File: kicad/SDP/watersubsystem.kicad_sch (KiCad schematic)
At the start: 6 parts

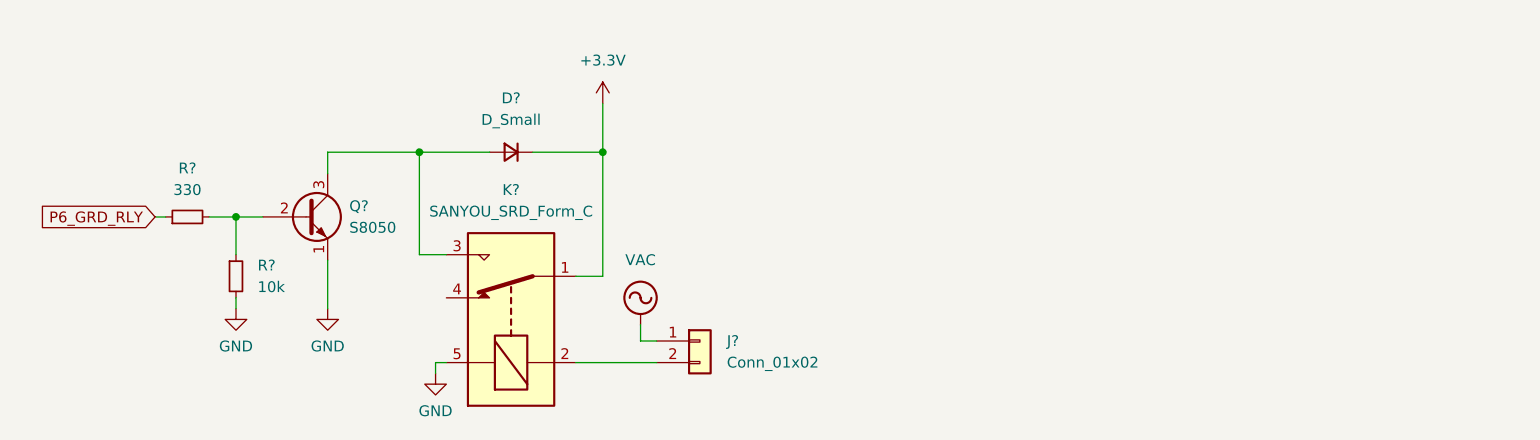
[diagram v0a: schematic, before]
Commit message: Updated schematics
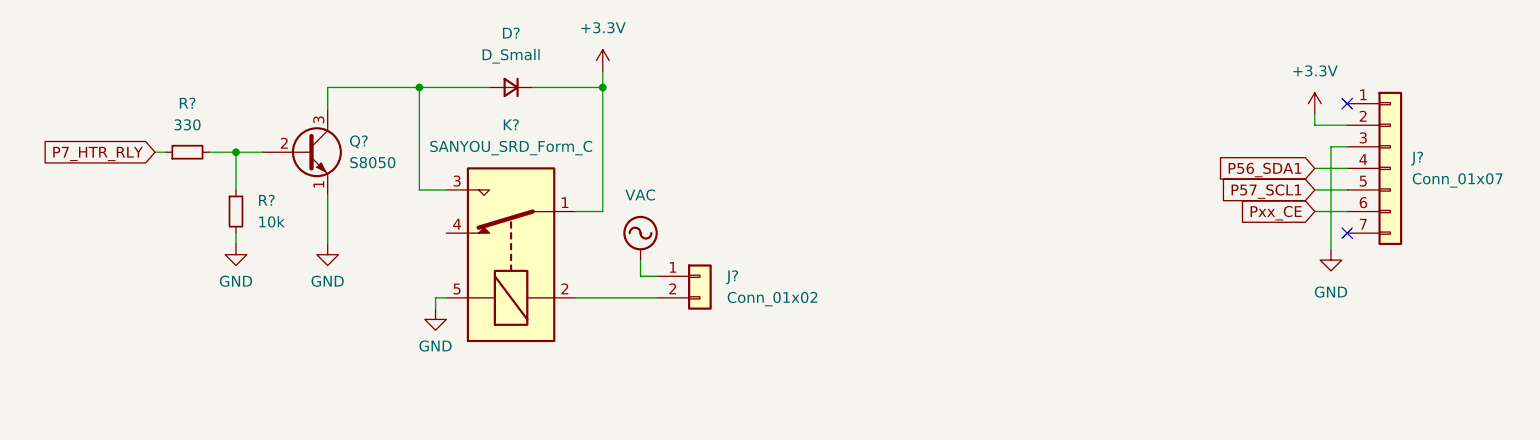
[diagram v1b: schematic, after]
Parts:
- removed D?: D_Small, symbol Device:D_Small
- removed J?: Conn_01x02, symbol Connector_Generic:Conn_01x02
- removed K?: SANYOU_SRD_Form_C, Relay_THT:Relay_SPDT_SANYOU_SRD_Series_Form_C, symbol Relay:SANYOU_SRD_Form_C
- removed Q?: S8050, Package_TO_SOT_THT:TO-92_Inline, symbol Transistor_BJT:S8050
- removed R?: 10k, symbol Device:R_Small
- removed R?: 330, symbol Device:R_Small
- added D?: D_Small, symbol Device:D_Small
- added J?: Conn_01x02, symbol Connector_Generic:Conn_01x02
- added J?: Conn_01x07, symbol Connector_Generic:Conn_01x07
- added K?: SANYOU_SRD_Form_C, Relay_THT:Relay_SPDT_SANYOU_SRD_Series_Form_C, symbol Relay:SANYOU_SRD_Form_C
- added Q?: S8050, Package_TO_SOT_THT:TO-92_Inline, symbol Transistor_BJT:S8050
- added R?: 330, symbol Device:R_Small
- added R?: 10k, symbol Device:R_Small
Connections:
- net +3V3: now also D?.1 (K), J?.2 (Pin_2), K?.1
- net GND: now also J?.3 (Pin_3), K?.5, Q?.1 (E), R?.2
- net VAC: now also J?.1 (Pin_1)
- new net: Q?.2 (B), R?.1, R?.2
- new net: D?.2 (A), K?.3, Q?.3 (C)
- new net: J?.2 (Pin_2), K?.2
- new net P56_SDA1: J?.4 (Pin_4)
- new net P57_SCL1: J?.5 (Pin_5)
- new net P7_HTR_RLY: R?.1
- new net Pxx_CE: J?.6 (Pin_6)
- no-connect marks 0 -> 2

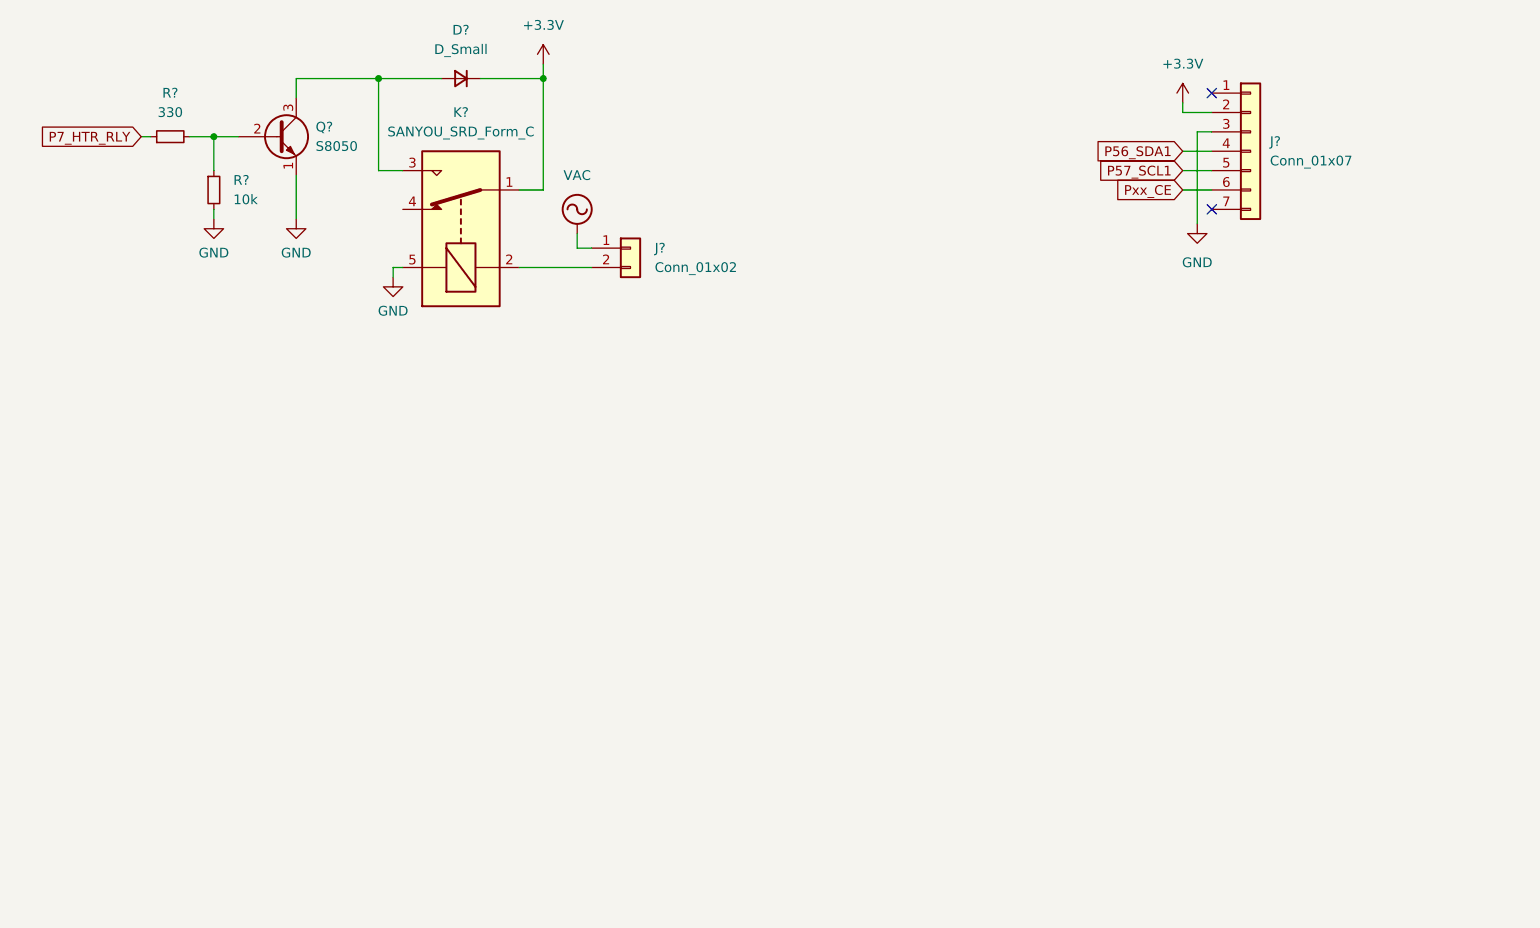
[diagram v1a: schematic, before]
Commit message: Updated schematics
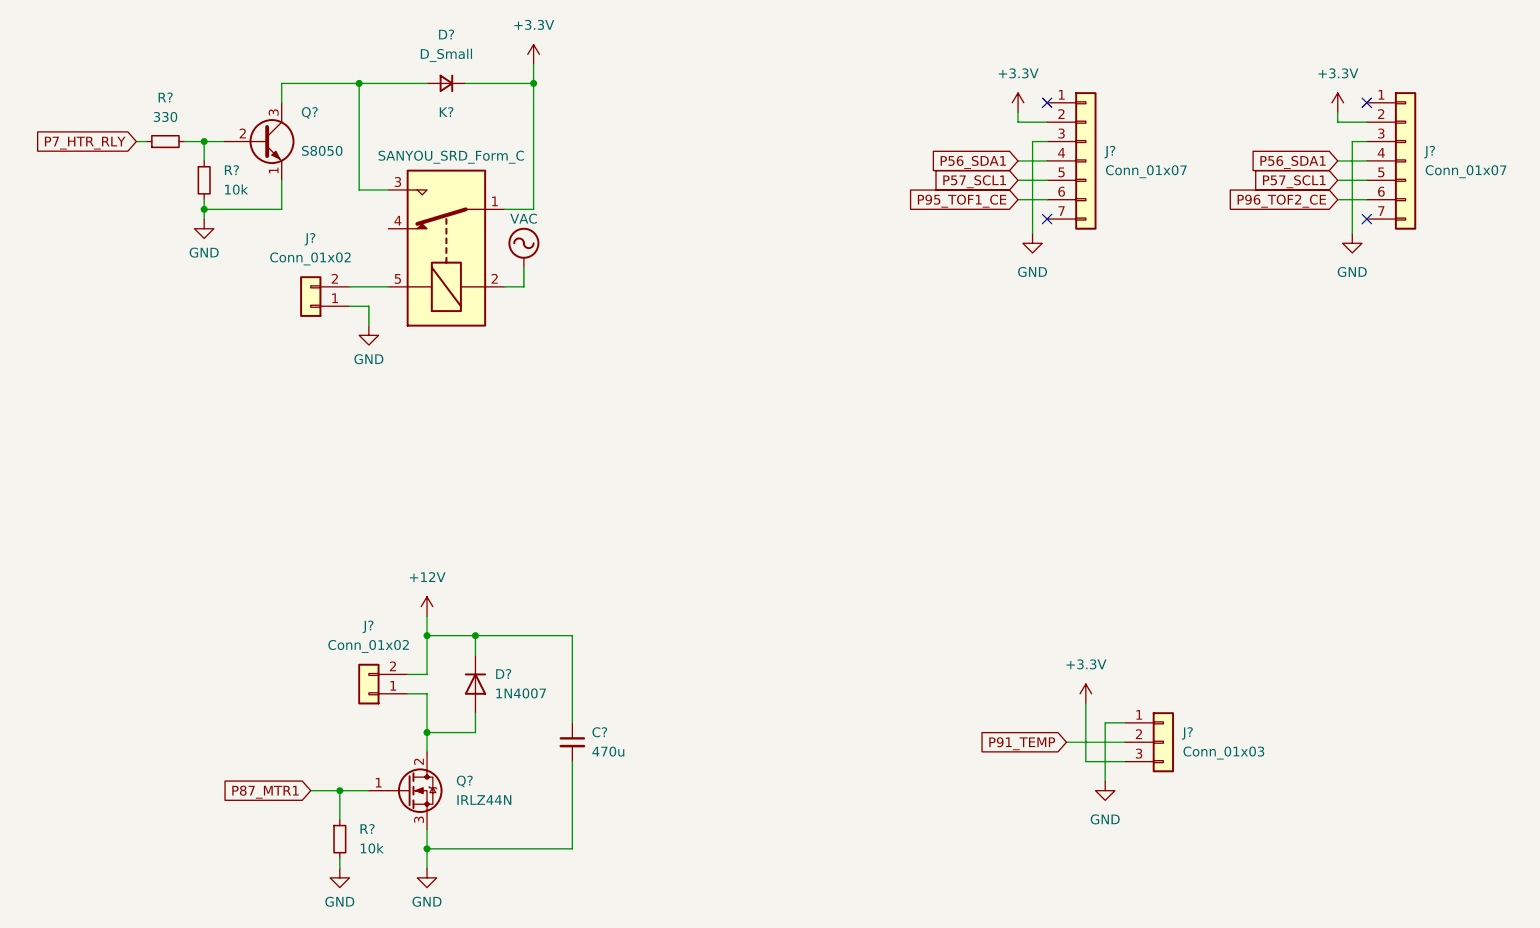
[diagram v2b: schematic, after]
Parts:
- added C?: 470u, symbol Device:C_Small
- added D?: 1N4007, Diode_THT:D_DO-41_SOD81_P10.16mm_Horizontal, symbol Diode:1N4007
- added J?: Conn_01x02, symbol Connector_Generic:Conn_01x02
- added J?: Conn_01x03, symbol Connector_Generic:Conn_01x03
- added J?: Conn_01x07, symbol Connector_Generic:Conn_01x07
- added Q?: IRLZ44N, Package_TO_SOT_THT:TO-220-3_Vertical, symbol Transistor_FET:IRLZ44N
- added R?: 10k, symbol Device:R_Small
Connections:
- net +3V3: now also J?.2 (Pin_2), J?.3 (Pin_3)
- net GND: now also J?.1 (Pin_1), C?.2, J?.1 (Pin_1), J?.3 (Pin_3), Q?.3 (S), R?.2; no longer K?.5
- net P56_SDA1: now also J?.4 (Pin_4)
- net P57_SCL1: now also J?.5 (Pin_5)
- net VAC: now also K?.2; no longer J?.1 (Pin_1)
- net at J?.2 (Pin_2): now also K?.5; no longer K?.2
- net Pxx_CE renamed P95_TOF1_CE
- new net: D?.2 (A), J?.1 (Pin_1), Q?.2 (D)
- new net +12V: C?.1, D?.1 (K), J?.2 (Pin_2)
- new net P87_MTR1: Q?.1 (G), R?.1
- new net P91_TEMP: J?.2 (Pin_2)
- new net P96_TOF2_CE: J?.6 (Pin_6)
- no-connect marks 2 -> 4
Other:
- moved on the sheet: D?, J?, K?, Q?, R?
